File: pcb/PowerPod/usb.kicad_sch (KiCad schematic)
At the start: 8 parts, among them IC2 FUSB302MPX, J1 GT-USB-7010, U1 SRV05-4

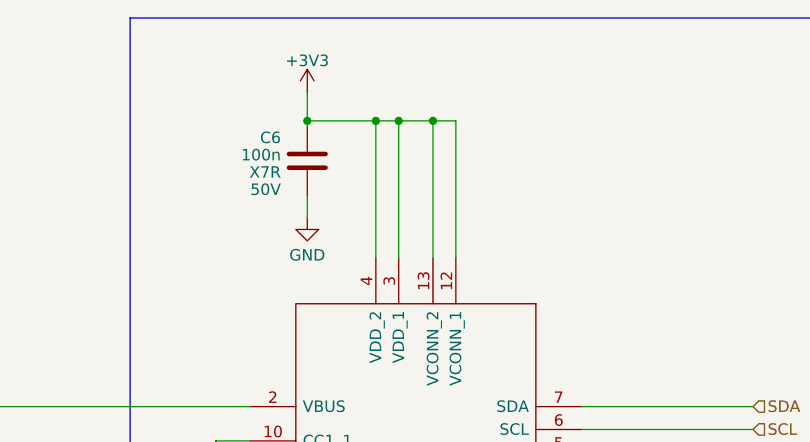
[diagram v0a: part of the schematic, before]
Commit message: finished layout
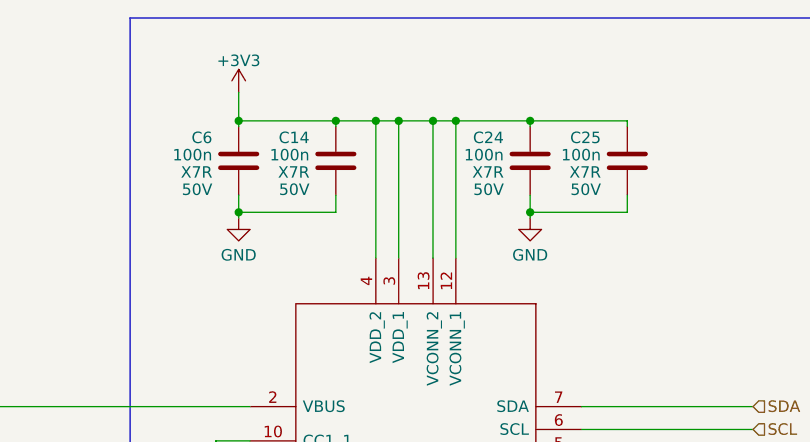
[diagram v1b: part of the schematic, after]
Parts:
- added C14, C24, C25: 100n, Capacitor_SMD:C_0402_1005Metric, symbol Capacitor_JLC:100n
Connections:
- net +3V3: now also C14.2, C24.2, C25.2
- net GND: now also C14.1, C24.1, C25.1
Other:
- moved on the sheet: C6
